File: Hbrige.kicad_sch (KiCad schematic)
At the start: 12 parts, among them J4 Conn_01x02

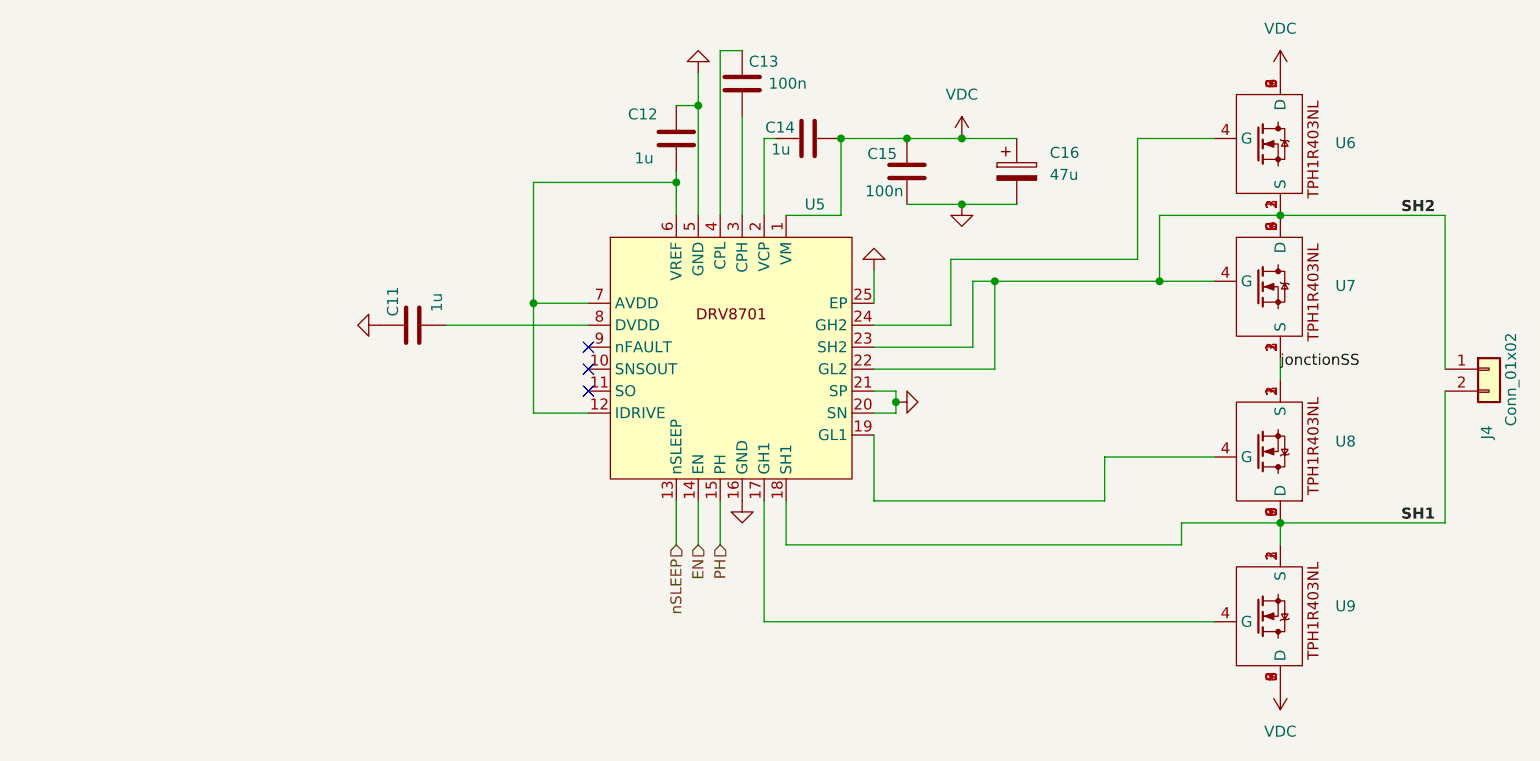
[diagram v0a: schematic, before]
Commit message: final push
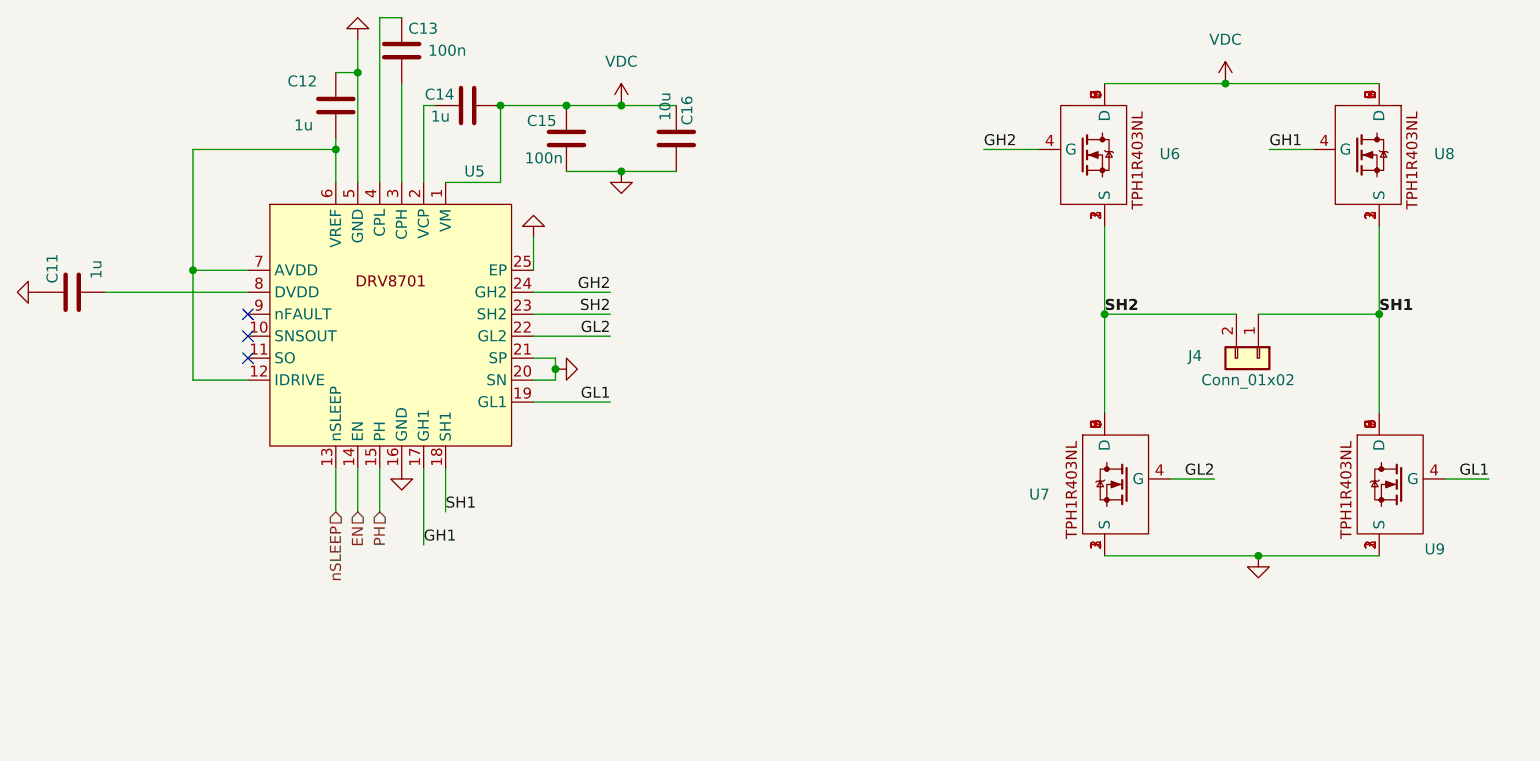
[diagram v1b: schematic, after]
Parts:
- removed C16: 47u, Capacitor:Wurth-47u-63V, symbol Device:C_Polarized
- added C16: 10u, Capacitor_SMD:C_0805_2012Metric, symbol Device:C
- renumbered U8 to U7, U7 to U8
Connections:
- net GND: now also U7.1 (S), U7.2 (S), U7.3 (S), U9.1 (S), U9.2 (S), U9.3 (S), C16.1
- net SH1: now also J4.1 (Pin_1), U8.1 (S), U8.2 (S), U8.3 (S), U9.5 (D), U9.6 (D), U9.7 (D), U9.8 (D), U9.9 (D); no longer J4.2 (Pin_2), U7.5 (D), U7.6 (D), U7.7 (D), U7.8 (D), U7.9 (D), U9.1 (S), U9.2 (S), U9.3 (S)
- net SH2: now also J4.2 (Pin_2), U7.5 (D), U7.6 (D), U7.7 (D), U7.8 (D), U7.9 (D); no longer J4.1 (Pin_1), U5.22 (GL2), U8.4 (G), U8.5 (D), U8.6 (D), U8.7 (D), U8.8 (D), U8.9 (D)
- net VDC: now also U8.5 (D), U8.6 (D), U8.7 (D), U8.8 (D), U8.9 (D), C16.2; no longer U9.5 (D), U9.6 (D), U9.7 (D), U9.8 (D), U9.9 (D)
- net GH2: now reaches U5.24 (GH2), U6.4 (G)
- net GH1: now reaches U5.17 (GH1)
- net GH1: now also U8.4 (G); no longer U9.4 (G)
- net GL1: now reaches U5.19 (GL1)
- net GL1: now also U9.4 (G); no longer U7.4 (G)
- removed net jonctionSS: U7.1 (S), U7.2 (S), U7.3 (S), U8.1 (S), U8.2 (S), U8.3 (S)
- new net GL2: U5.22 (GL2), U7.4 (G)
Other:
- moved on the sheet: C11, C12, C13, C14, C15, J4, U5, U6, U7, U8, U9
